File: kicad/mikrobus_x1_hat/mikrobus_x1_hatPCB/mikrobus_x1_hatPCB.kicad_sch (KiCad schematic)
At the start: 2 parts, among them IC1 MIKROE-924, J1 RPi_GPIO

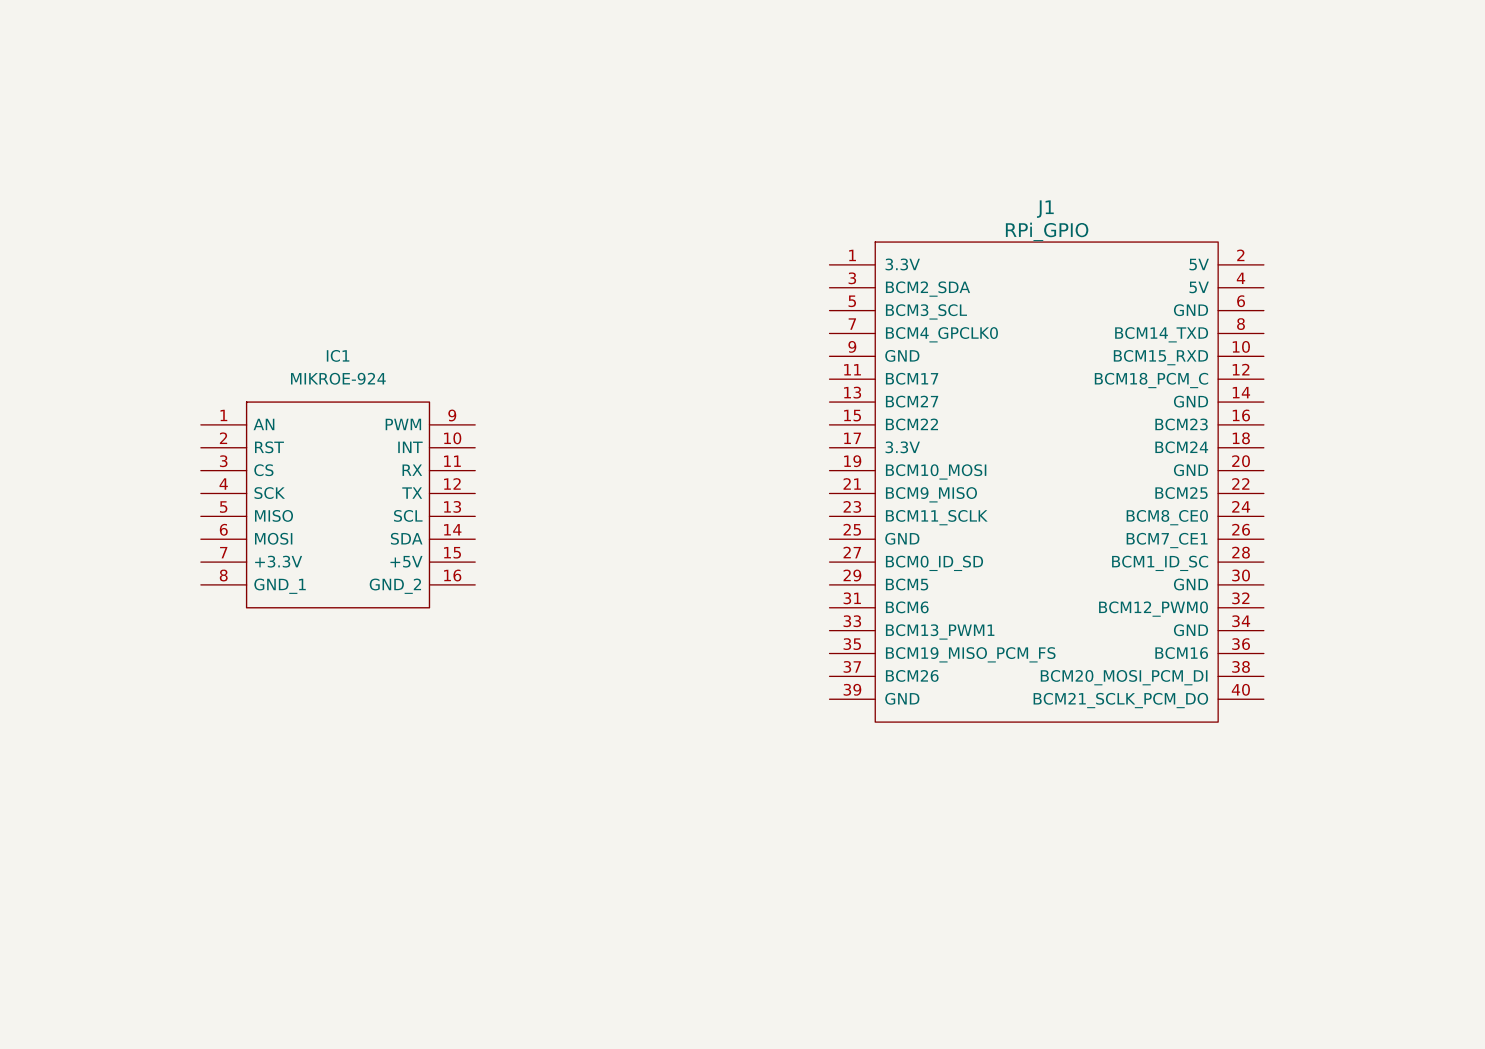
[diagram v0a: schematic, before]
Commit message: schematic complete with 0 ERC errors
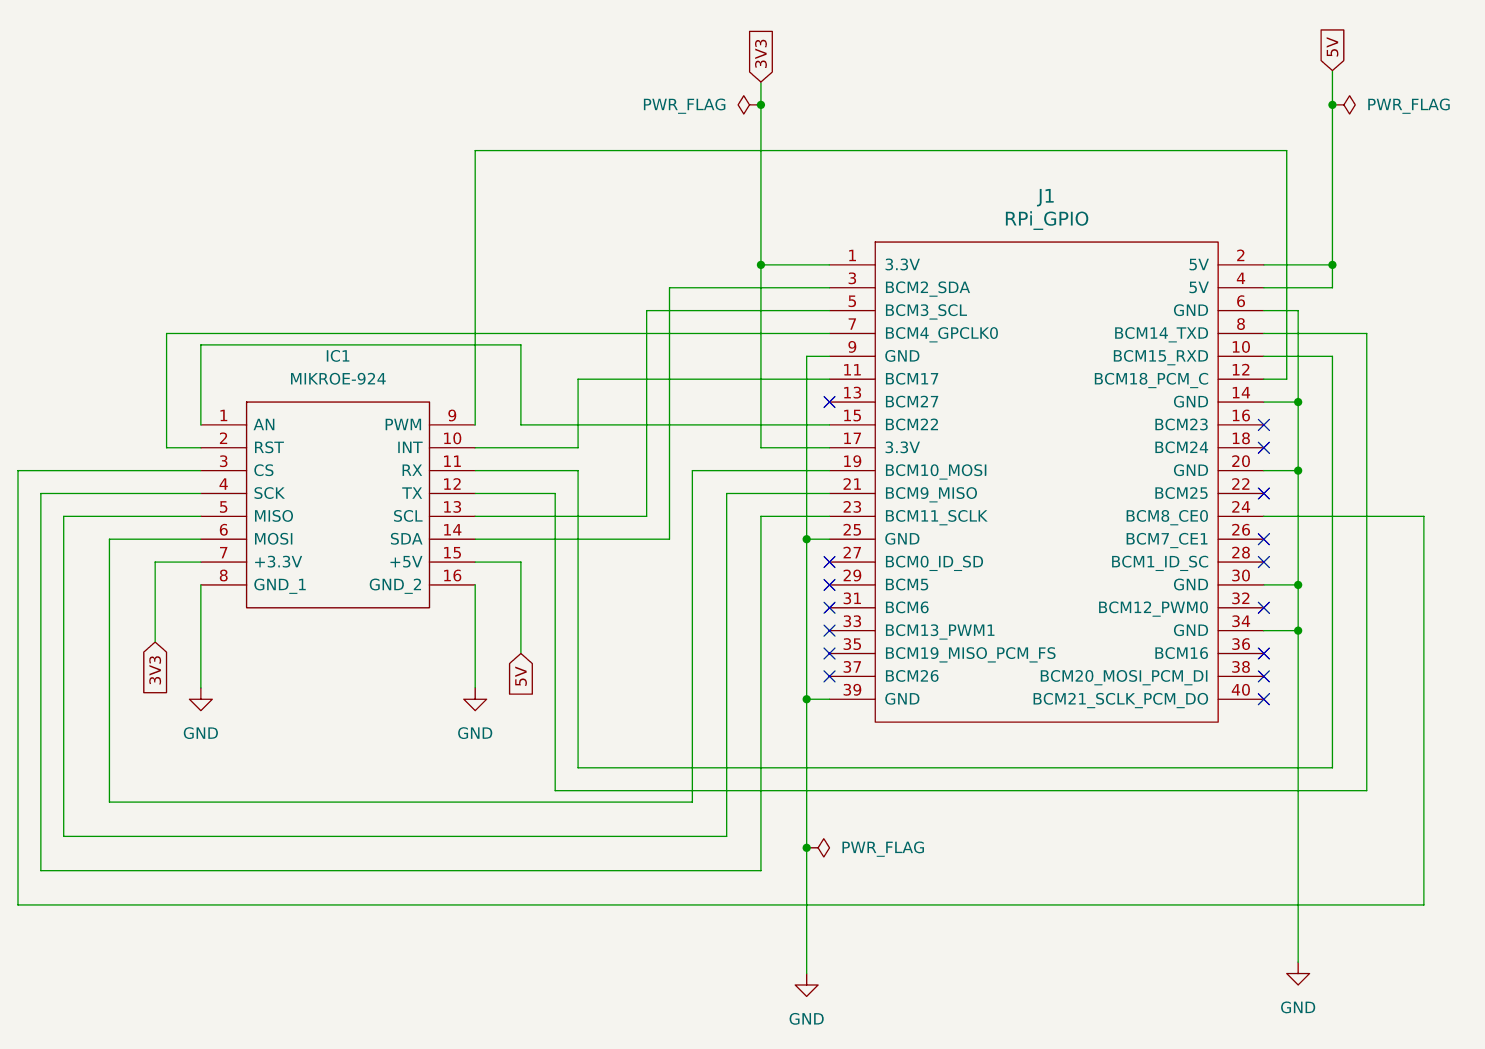
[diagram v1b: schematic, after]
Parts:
- removed J1: RPi_GPIO, RPi_Hat:Pin_Header_Straight_2x20, symbol RPi_Hat:RPi_GPIO
- added J1: RPi_GPIO, symbol RPi_HAT:RPi_GPIO
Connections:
- net at IC1.1 (AN): now also J1.15 (BCM22)
- net at IC1.10 (INT): now also J1.11 (BCM17)
- net at IC1.11 (RX): now also J1.10 (BCM15_RXD)
- net at IC1.12 (TX): now also J1.8 (BCM14_TXD)
- net at IC1.13 (SCL): now also J1.5 (BCM3_SCL)
- net at IC1.14 (SDA): now also J1.3 (BCM2_SDA)
- net 5V: now reaches IC1.15 (+5V)
- net 5V: now also J1.2 (5V), J1.4 (5V)
- net GND: now reaches IC1.16 (GND_2)
- net GND: now also IC1.8 (GND_1), J1.14 (GND), J1.20 (GND), J1.25 (GND), J1.30 (GND), J1.34 (GND), J1.39 (GND), J1.6 (GND), J1.9 (GND)
- net at IC1.2 (RST): now also J1.7 (BCM4_GPCLK0)
- net at IC1.3 (CS): now also J1.24 (BCM8_CE0)
- net at IC1.4 (SCK): now also J1.23 (BCM11_SCLK)
- net at IC1.5 (MISO): now also J1.21 (BCM9_MISO)
- net at IC1.6 (MOSI): now also J1.19 (BCM10_MOSI)
- net 3V3: now reaches IC1.7 (+3.3V)
- net 3V3: now also J1.1 (3.3V), J1.17 (3.3V)
- net at IC1.9 (PWM): now also J1.12 (BCM18_PCM_C)
- no-connect marks 0 -> 16
